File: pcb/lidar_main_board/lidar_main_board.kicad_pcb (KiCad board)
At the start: 2 copper layers, 70 x 50 mm, 27 parts, among them J1 vl53l1x, J2 AS5600, J3 HC-06, J4 Bateria, J5 Boton 1, J6 Boton 2, J7 Boton 3, J8 Motor, U1 LPC845-BRK, U2 AMS1117-3.3, U3 LM7805_TO220

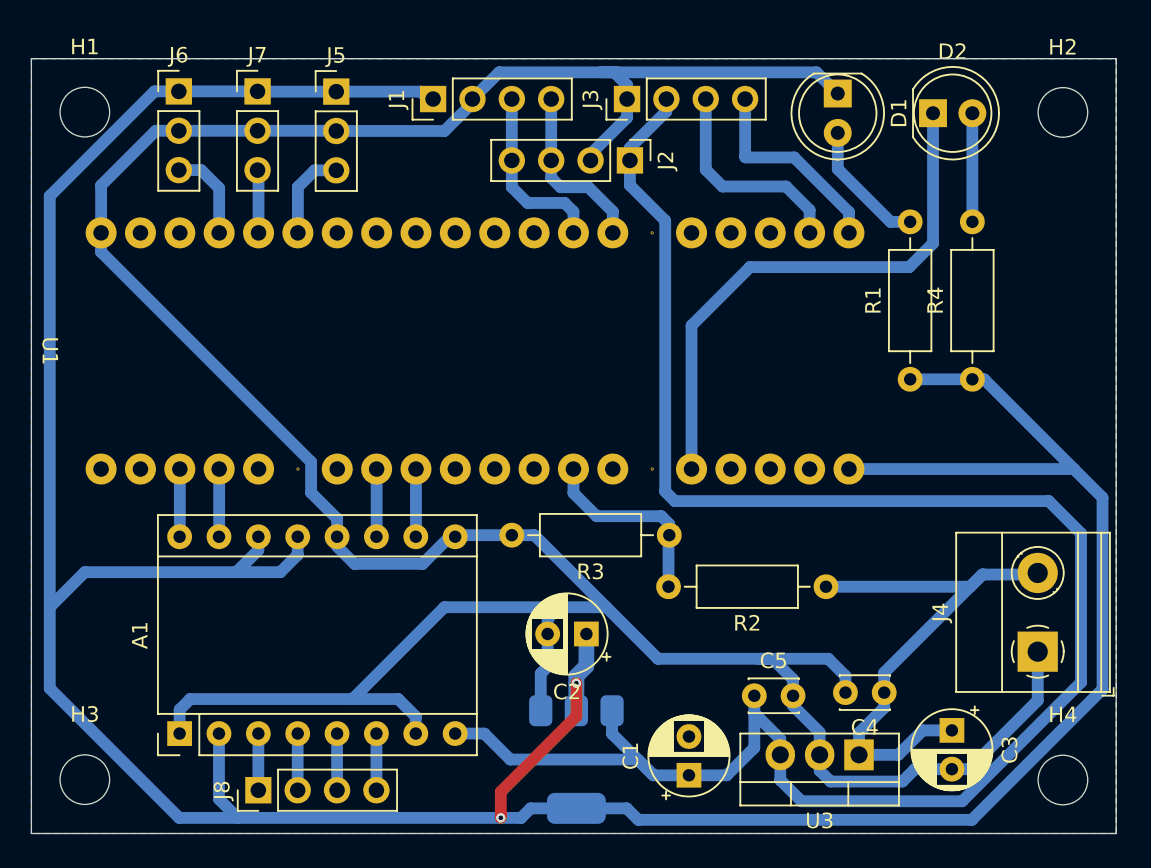
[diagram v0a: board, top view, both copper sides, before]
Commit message: new version pcb
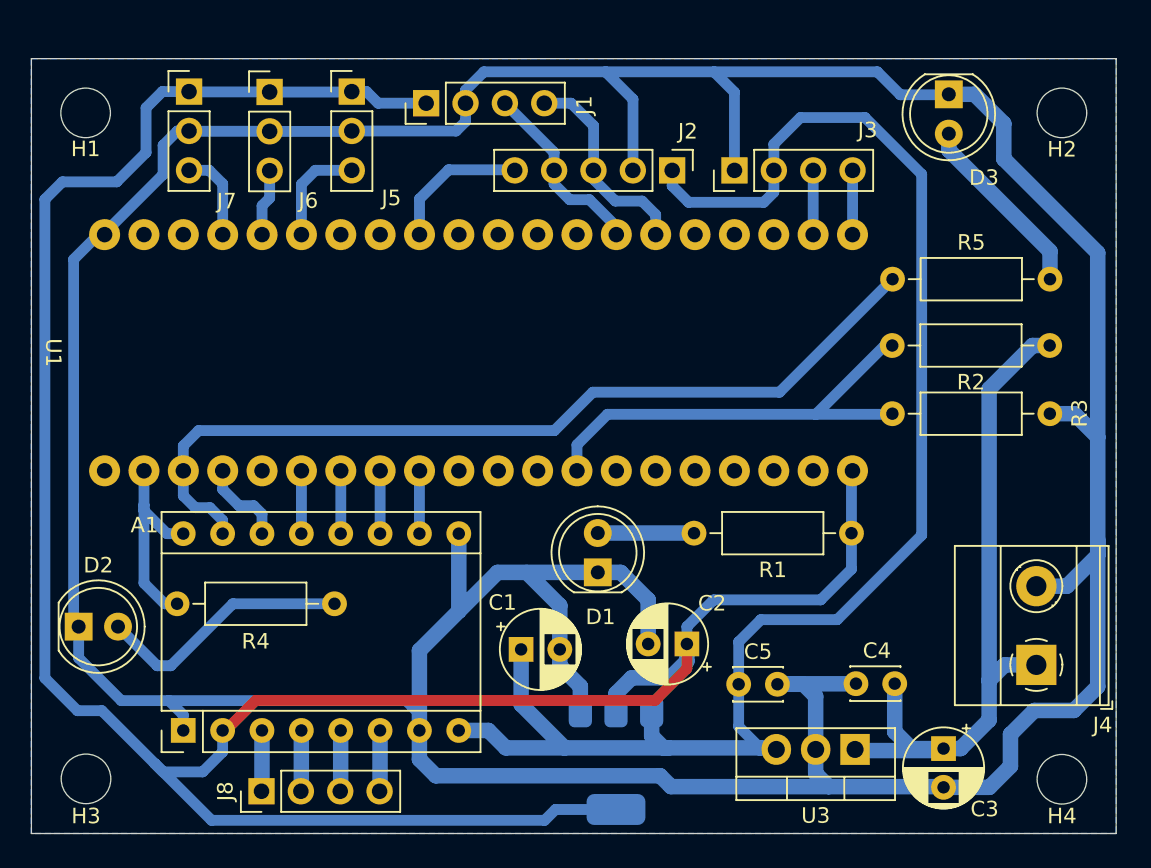
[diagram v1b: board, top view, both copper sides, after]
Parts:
- added D3: LED, LED_THT:LED_D5.0mm, F.Cu at (79.2, 22.3)
- added R5: 120, Resistor_THT:R_Axial_DIN0207_L6.3mm_D2.5mm_P10.16mm_Horizontal, F.Cu at (75.6, 34.2)
- D1: value LED_PWR -> LED
- J2: footprint Connector_PinHeader_2.54mm:PinHeader_1x04_P2.54mm_Vertical -> Connector_PinHeader_2.54mm:PinHeader_1x05_P2.54mm_Vertical
- moved D2 64.3 mm to (23.1, 56.6)
- moved R4 53.3 mm to (29.4, 55.2), turned to 0 degrees
- moved D1 34.6 mm to (56.5, 53.1), turned to 90 degrees
- moved R2 21.2 mm to (85.7, 38.5)
- moved R3 16.4 mm to (75.6, 42.9), turned to 0 degrees
- moved C1 13.5 mm to (51.6, 58.1), turned to 0 degrees
- moved R1 10.6 mm to (72.9, 50.6), turned to 180 degrees
- moved J3 8.32 mm to (65.4, 27.2)
- moved C2 6.52 mm to (62.3, 57.8)
- moved J6 5.86 mm to (35.4, 22.1)
- moved J7 4.42 mm to (30.2, 22.1)
- moved J2 2.80 mm to (61.4, 27.2)
- moved U2 2.56 mm to (57.7, 65.3)
- moved C3 1.29 mm to (78.9, 64.5)
- moved C5 1.25 mm to (65.6, 60.4)
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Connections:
- A1 pad 12: GND -> MS3
- A1 pad 13: +3V3 -> MRESET
- A1 pad 14: +3V3 -> MSLEEP
- D2 pad 1: LED_DIR -> GND
- J4 pad 1: GND -> +BATT
- J4 pad 2: +BATT -> GND
- R4 pad 1: +3V3 -> DIR
- U1 pad 12: unconnected-(U1-PIO0_26-Pad12) -> DIR_AS5600
- U1 pad 16: BTN_SEL -> BTN_MODE
- U1 pad 17: BTN_MODE -> BTN_SEL
- U1 pad 22: unconnected-(U1-PIO0_09-Pad22) -> DIR
- U1 pad 23: DIR -> STEP
- U1 pad 24: STEP -> MSLEEP
- U1 pad 26: unconnected-(U1-PIO0_13-Pad26) -> MRESET
- U1 pad 27: unconnected-(U1-PIO0_14-Pad27) -> MS3
- U1 pad 36: LED_DIR -> unconnected-(U1-PIO0_03_SWCLK-Pad36)
- U1 pad 6: unconnected-(U1-PIO0_21-Pad6) -> I2C1 - SCL
- U1 pad 7: I2C1 - SCL -> I2C1 - SDA
- U1 pad 8: I2C1 - SDA -> unconnected-(U1-PIO0_23-Pad8)
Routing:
- net GND: track 201.3 -> 289.3 mm
- net STEP: track 4.37 -> 57.5 mm
- net +3V3: track 221.0 -> 168.5 mm, vias 2 -> 0
- net LED_DIR: track 35.4 -> 0.00 mm
- net +5V: track 122.8 -> 100.0 mm
- net BAT_ADC: track 12.6 -> 29.6 mm
- net Net-(D3-A): track 0.00 -> 12.1 mm
- net +BATT: track 35.6 -> 46.1 mm
- net UART0 - RX: track 13.8 -> 4.15 mm
- net Net-(D2-A): track 7.01 -> 16.7 mm
- net DIR: track 4.37 -> 13.9 mm
- net DIR_AS5600: track 0.00 -> 9.24 mm
- net UART0 - TX: track 13.2 -> 4.15 mm
- net MSLEEP: track 0.00 -> 5.66 mm
- net MS3: track 0.00 -> 4.06 mm
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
